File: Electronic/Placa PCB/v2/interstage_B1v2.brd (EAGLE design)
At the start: 82.5 x 29 mm, 7 parts, among them Q1 PMV16XNR, U1 MCP9808T-E/MS, U3 MCP9808T-E/MS

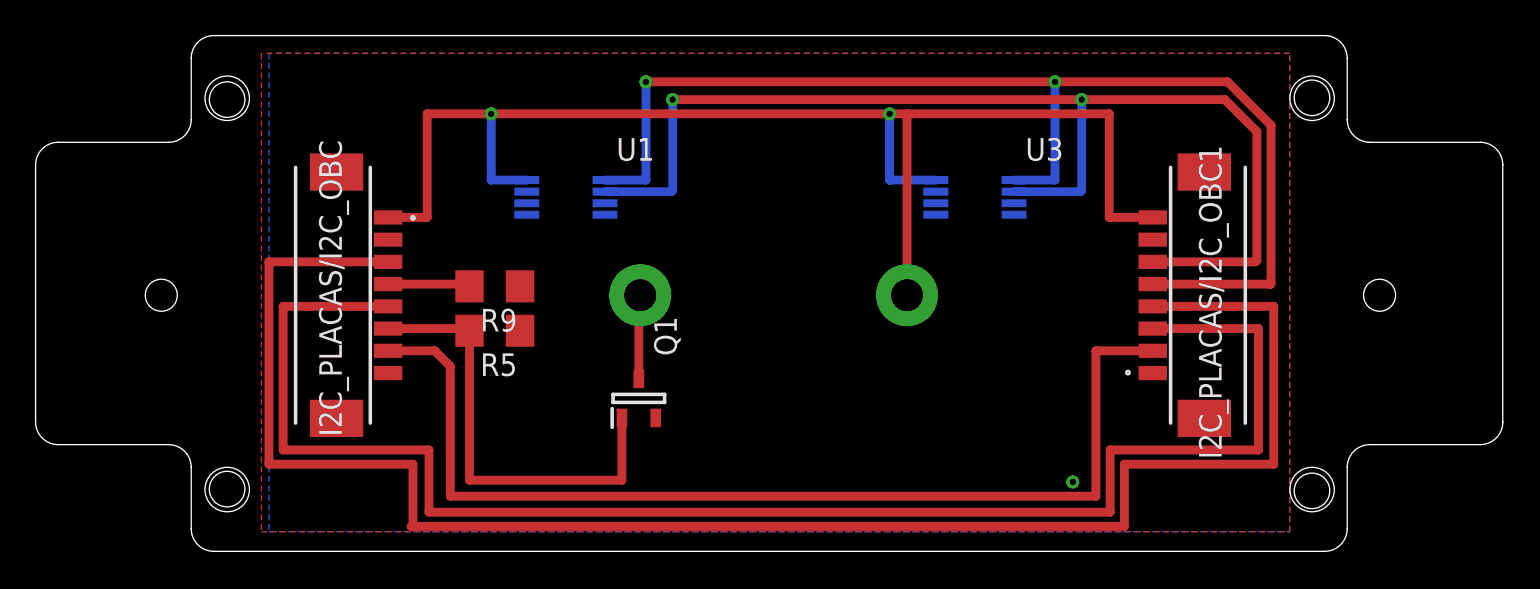
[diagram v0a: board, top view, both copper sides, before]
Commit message: Placas PCB
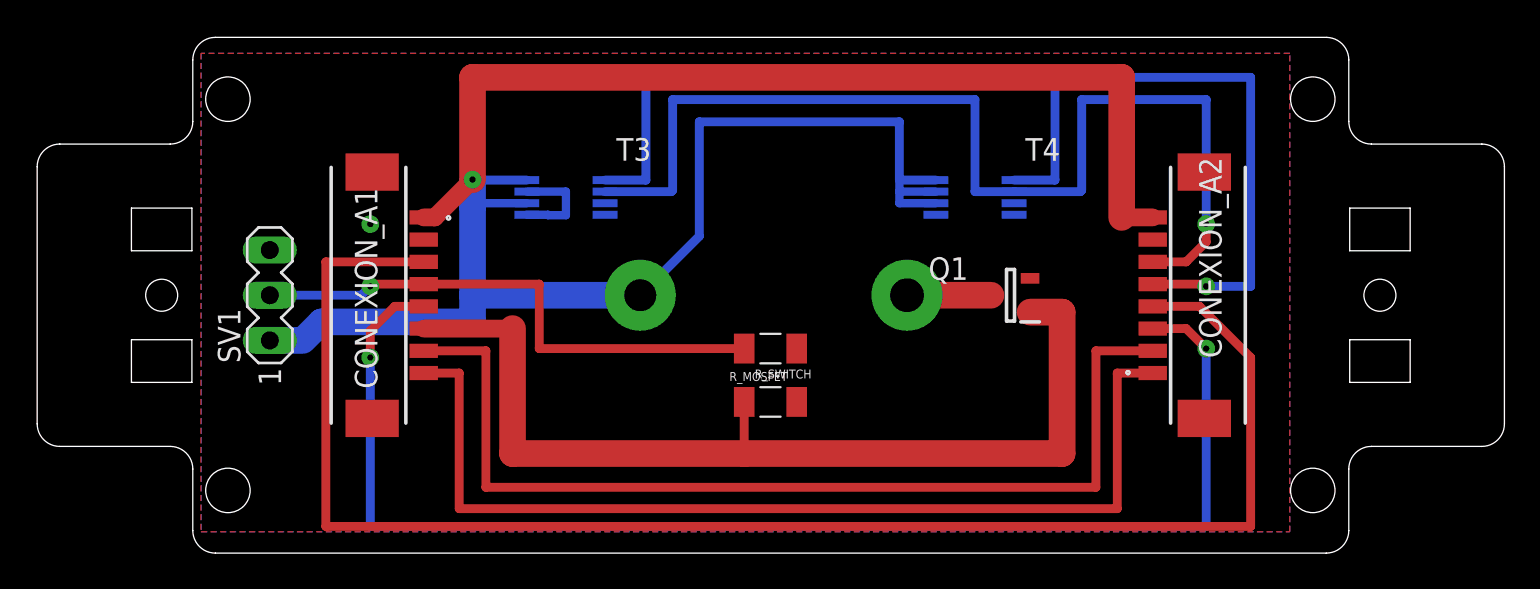
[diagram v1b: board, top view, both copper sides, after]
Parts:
- removed I2C_PLACAS/I2C_OBC: 53261-0871, SamacSys_Parts:53261-0871
- removed R5, R9: 330 Ohm, rcl:R1206
- added CONEXION_A1: 53261-0871, SamacSys_Parts:53261-0871
- added R_MOSFET, R_SWITCH: ERA-8AEB331V, resistor_330_smd:RESC3216X70N
- added SV1: (no value), con-lstb:MA03-1
- moved Q1 21.7 mm to (46.0, 14.5), turned to 180 degrees
- renumbered I2C_PLACAS/I2C_OBC1 to CONEXION_A2, U1 to T3, U3 to T4
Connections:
- net MOSFET renamed NICROMO
- removed net N$4: R9.1
- net AIN0: now also CONEXION_A1.5; no longer I2C_PLACAS/I2C_OBC.5
- net AIN1: now also CONEXION_A1.4, R_SWITCH.2, SV1.2; no longer I2C_PLACAS/I2C_OBC.4, R9.2
- net GND: now also CONEXION_A1.2, R_MOSFET.2, R_SWITCH.1, T3.5, T3.7, T4.5; no longer I2C_PLACAS/I2C_OBC.2, R5.1
- net INT0: now also CONEXION_A1.7; no longer I2C_PLACAS/I2C_OBC.7
- net OC1A: now also CONEXION_A1.3; no longer I2C_PLACAS/I2C_OBC.3
- net T0: now also CONEXION_A1.8
- net T1: now also CONEXION_A1.6, R_MOSFET.1; no longer I2C_PLACAS/I2C_OBC.6, R5.2
- net VCC: now also CONEXION_A1.1, SV1.1, T3.6, T4.6, T4.7; no longer I2C_PLACAS/I2C_OBC.1
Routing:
- net T0: track 0.00 -> 56.2 mm
- net VCC: track 76.9 -> 124.0 mm, vias 3 -> 2
- net T1: track 25.1 -> 55.6 mm
- net AIN1: track 4.63 -> 30.6 mm, vias 0 -> 1
- net AIN0: track 88.6 -> 75.0 mm, vias 0 -> 2
- net OC1A: track 97.4 -> 88.6 mm
- net GND: track 0.00 -> 5.75 mm
- net SCL: track 64.6 -> 60.7 mm, vias 2 -> 1
- net INT0: track 58.8 -> 56.3 mm
- net SDA: track 67.4 -> 67.5 mm, vias 2 -> 1
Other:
- outline, holes or cut-outs redrawn
